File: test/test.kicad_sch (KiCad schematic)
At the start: 22 parts, among them J1 Conn_01x02, J2 Conn_01x02, J3 Conn_01x10, U1 DRV8873SPWPRQ1

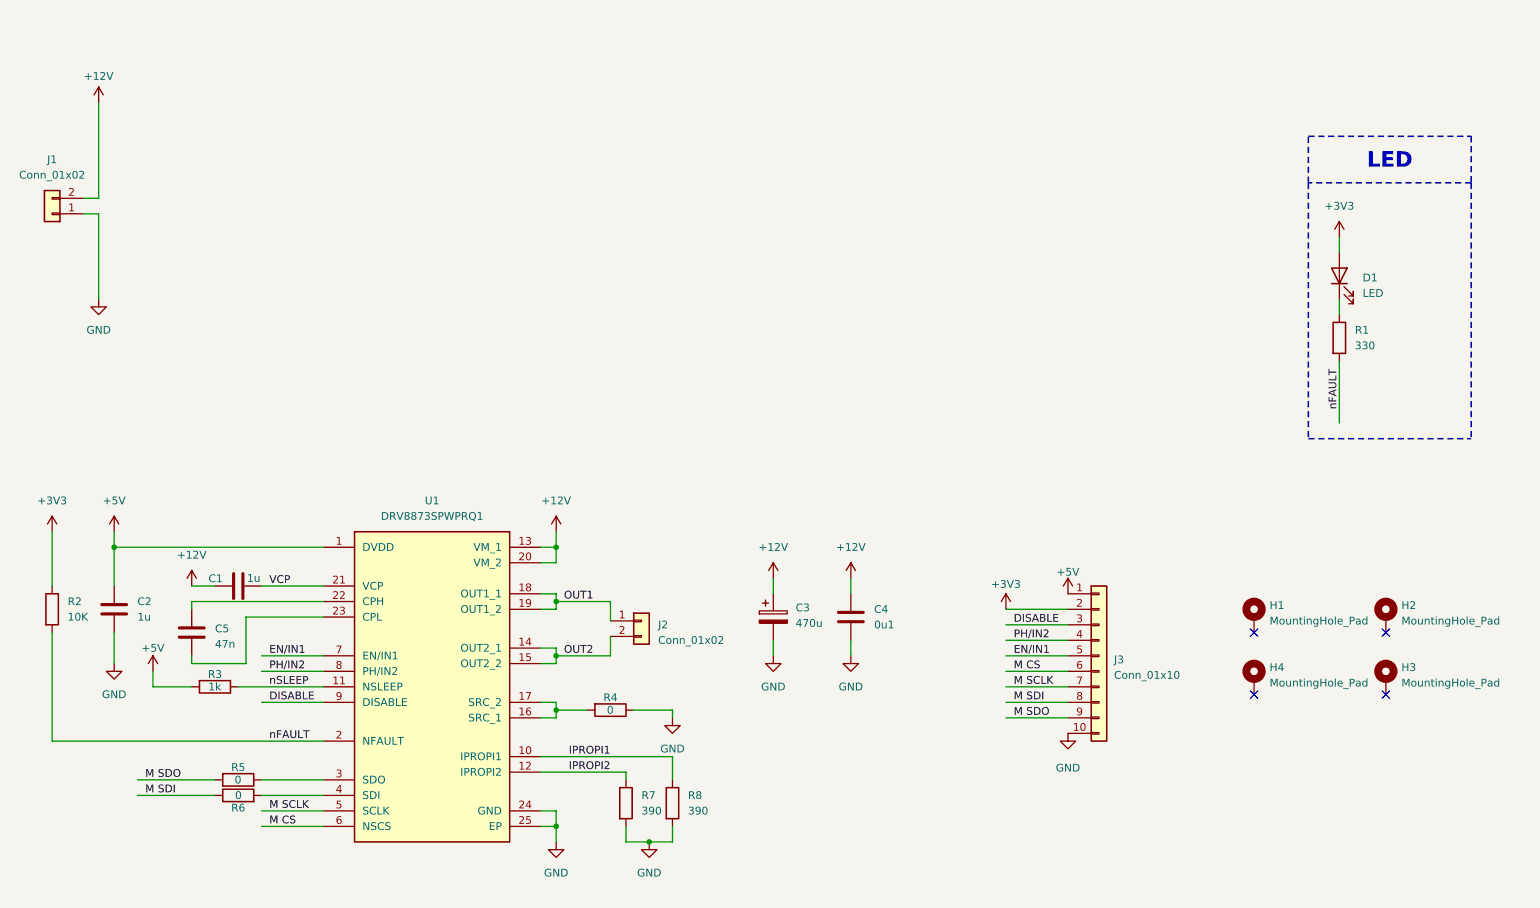
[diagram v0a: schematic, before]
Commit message: Schematic Formatting
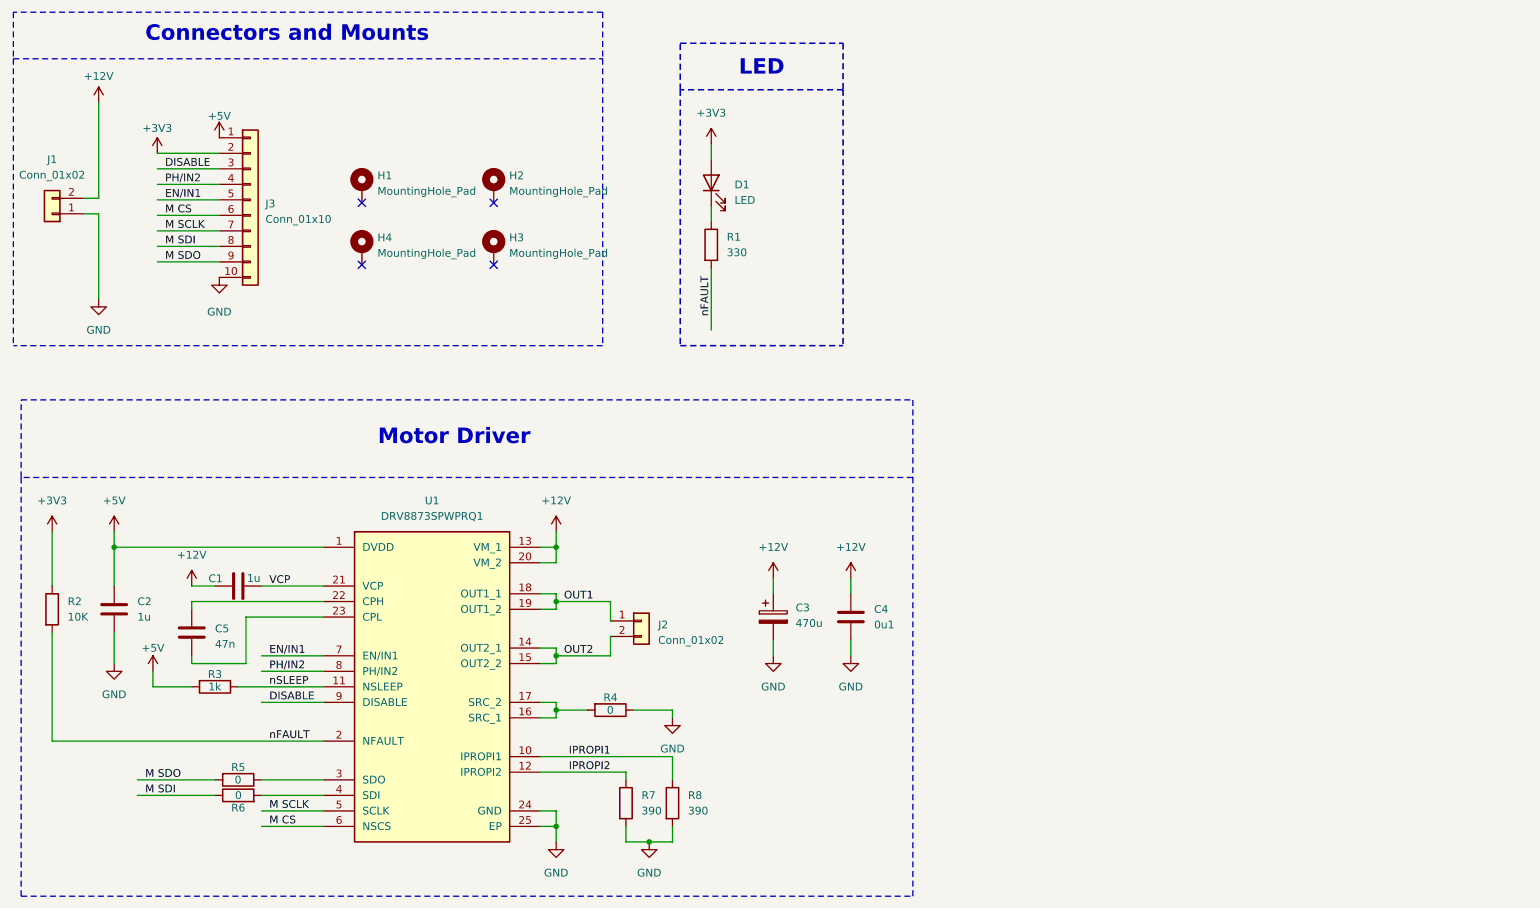
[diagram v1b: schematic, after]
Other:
- note added: "Connectors and Mounts"
- note added: "Motor Driver"
- moved on the sheet: D1, H1, H2, H3, H4, J3, R1
